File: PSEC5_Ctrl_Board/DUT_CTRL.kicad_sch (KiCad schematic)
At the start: 2 parts, among them J2 QSH-040-01-X-D-DP-A, J4 QSH-040-01-X-D-DP-A

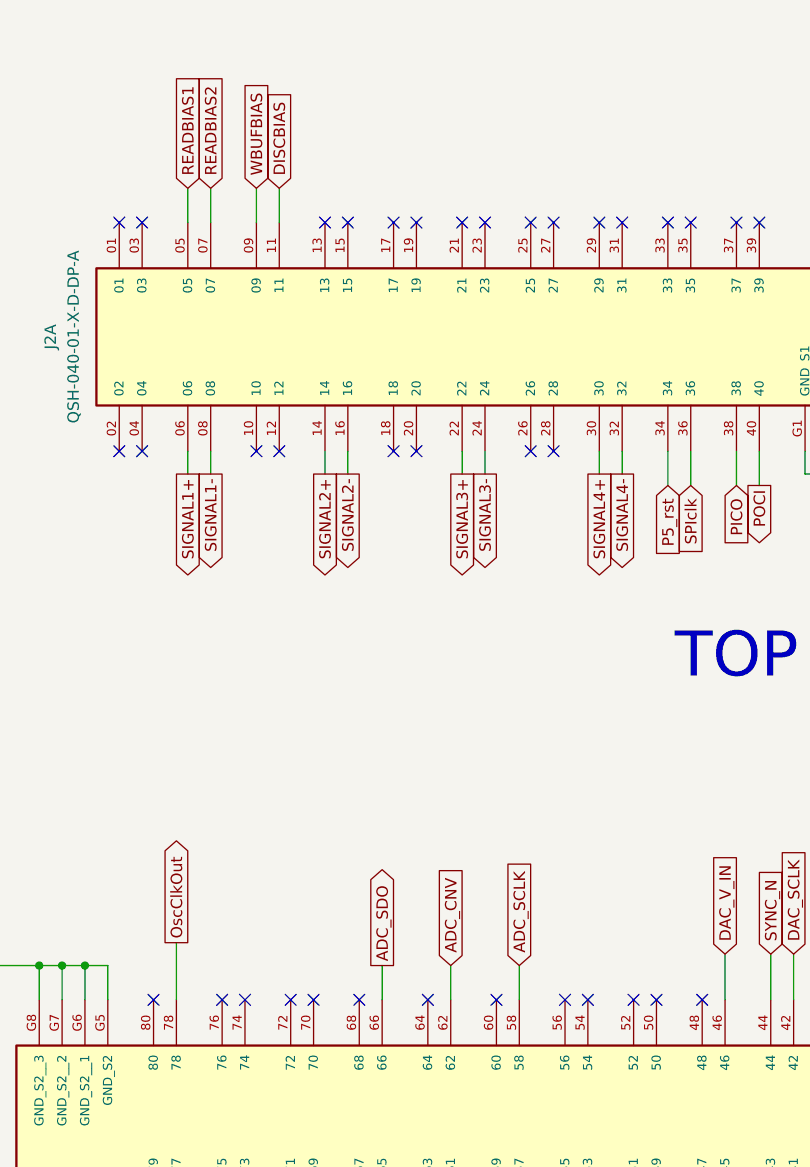
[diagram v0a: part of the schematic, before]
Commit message: Changes
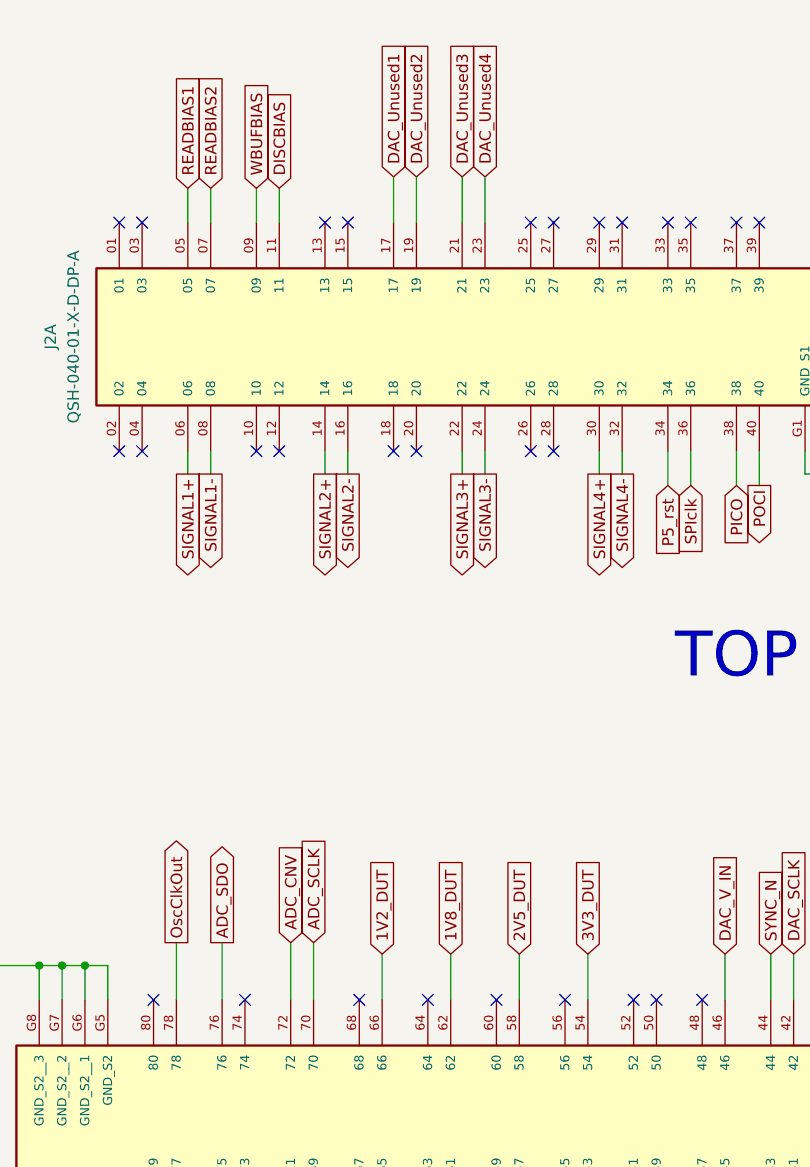
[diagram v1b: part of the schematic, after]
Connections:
- net ADC_CNV: now also J4.72; no longer J4.62
- net ADC_SCLK: now also J4.70; no longer J4.58
- net ADC_SDO: now also J4.76; no longer J4.66
- net DAC_Unused1: now reaches J2.17
- net DAC_Unused2: now reaches J2.19
- net DAC_Unused3: now reaches J2.21
- net DAC_Unused4: now reaches J2.23
- net 3V3_DUT: now reaches J4.54
- new net 1V2_DUT: J4.66
- new net 1V8_DUT: J4.62
- new net 2V5_DUT: J4.58
- no-connect marks 59 -> 51

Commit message: My PC is fading, pushing in case it dies
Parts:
- J2, J4: footprint QSH-040-01-X-D-DP-A:SAMTEC_QSH-040-01-X-D-DP-A -> QSH-040-01-L-D-DP-A:SAMTEC_QSH-040-01-X-D-DP-A
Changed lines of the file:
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@@
 			)
 		)
-		(property "Footprint" "QSH-040-01-X-D-DP-A:SAMTEC_QSH-040-01-X-D-DP-A"
+		(property "Footprint" "QSH-040-01-L-D-DP-A:SAMTEC_QSH-040-01-X-D-DP-A"
 			(at 59.69 54.102 0)
 			(effects
@@
 			)
 		)
-		(property "Footprint" "QSH-040-01-X-D-DP-A:SAMTEC_QSH-040-01-X-D-DP-A"
+		(property "Footprint" "QSH-040-01-L-D-DP-A:SAMTEC_QSH-040-01-X-D-DP-A"
 			(at 158.75 52.832 0)
 			(effects
@@
 			)
 		)
-		(property "Footprint" "QSH-040-01-X-D-DP-A:SAMTEC_QSH-040-01-X-D-DP-A"
+		(property "Footprint" "QSH-040-01-L-D-DP-A:SAMTEC_QSH-040-01-X-D-DP-A"
 			(at 147.32 128.778 0)
 			(effects
@@
 			)
 		)
-		(property "Footprint" "QSH-040-01-X-D-DP-A:SAMTEC_QSH-040-01-X-D-DP-A"
+		(property "Footprint" "QSH-040-01-L-D-DP-A:SAMTEC_QSH-040-01-X-D-DP-A"
 			(at 248.92 130.048 0)
 			(effects
